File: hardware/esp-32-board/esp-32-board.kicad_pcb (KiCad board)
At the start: 2 copper layers, 53.8 x 69.1 mm, 38 parts, among them J1 MainConnector, J2 Conn_01x06, J3 ESP-PROG-Program, J4 ESP-PROG-Debug, J5 USB_B_Micro, J6 Barrel_Jack_MountingPin, J7 Conn_01x02, Q1 BCR129S, SW1 SW_Push, SW2 SW_Push, U1 ESP32-WROOM-32, U2 USBLC6-2SC6, U3 FT232RL, U4 NCP1117ST50T3G, U5 NCP1117-3.3

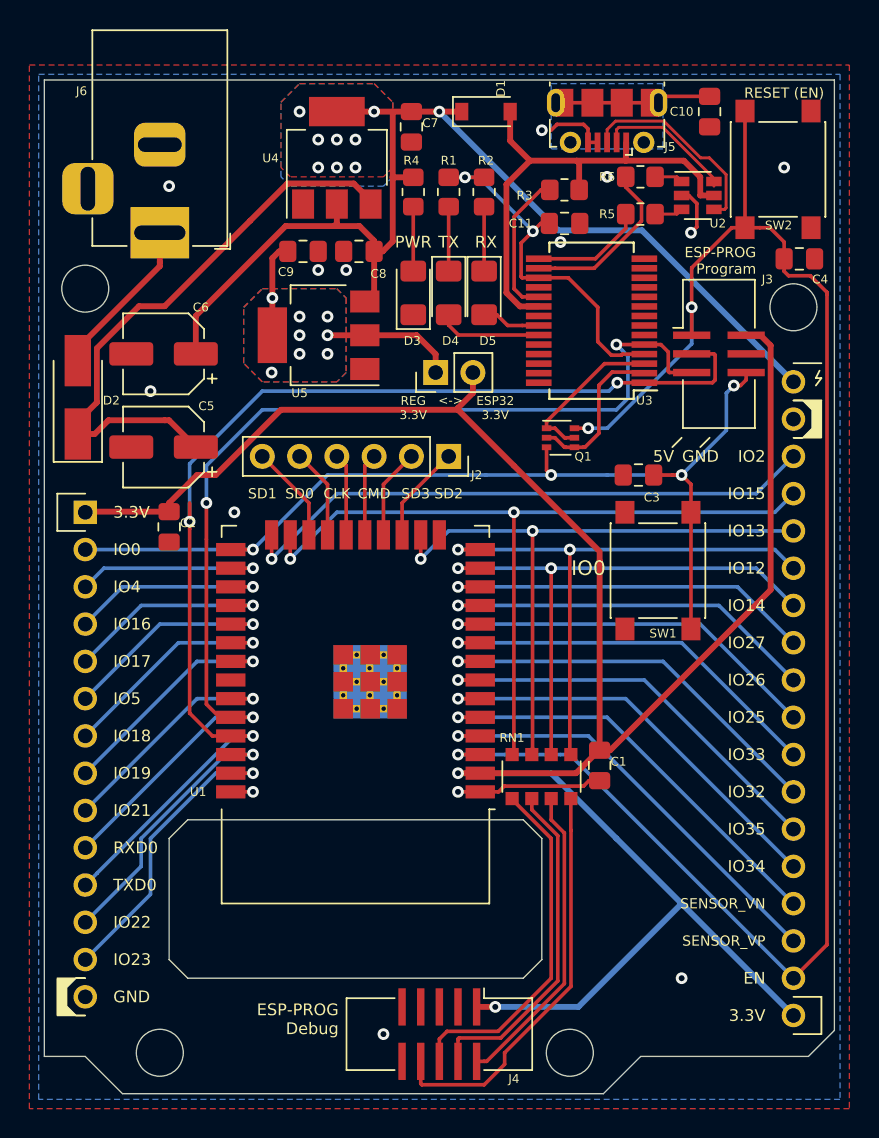
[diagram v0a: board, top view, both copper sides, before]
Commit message: Cleanup tracks and vias
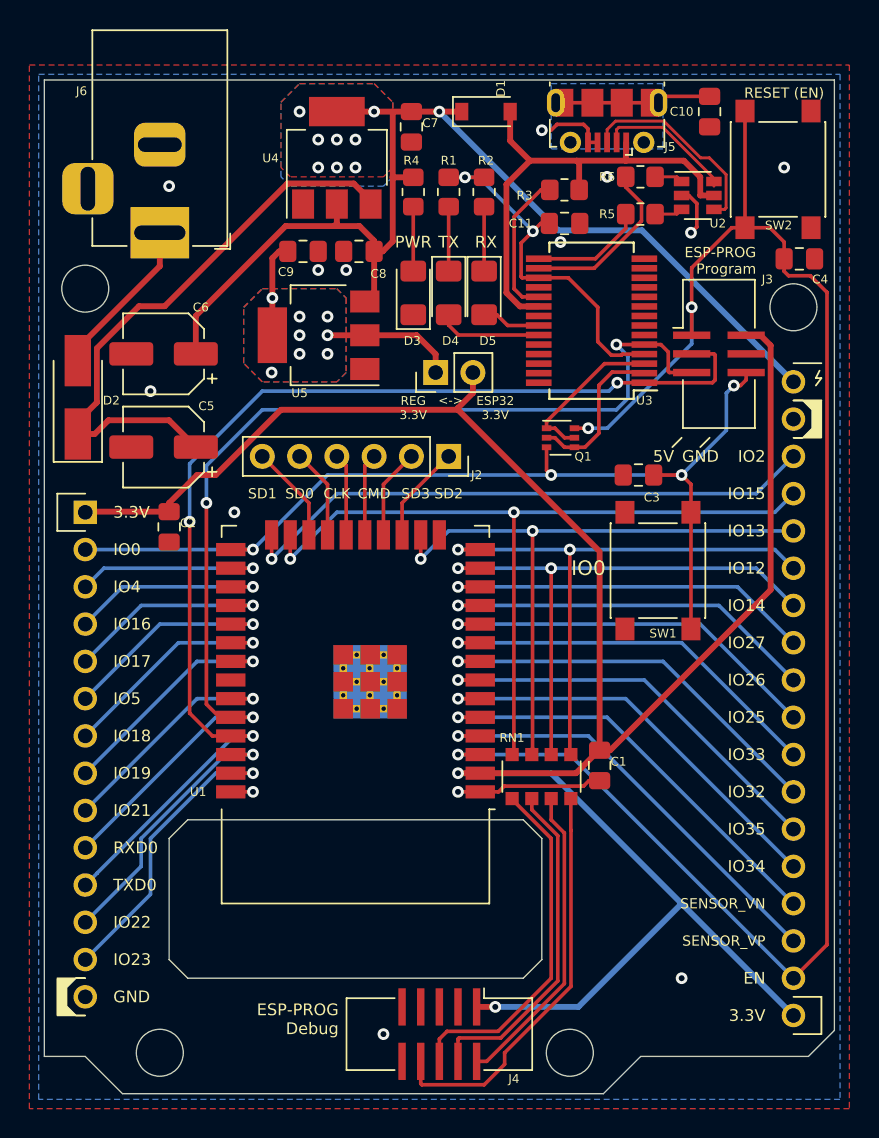
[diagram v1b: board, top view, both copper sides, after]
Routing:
- net /TXD0: track 80.4 -> 79.1 mm
